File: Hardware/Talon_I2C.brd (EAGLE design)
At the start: 140 x 19 mm, 88 parts, among them J1 CONN_TALON_REMOTE, J2 CONN_SDI-12_LOGGERM8_TE_BOARD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, J3 CONN_SDI-12_LOGGERM8_TE_BOARD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, J4 CONN_SDI-12_LOGGERM8_TE_BOARD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, J5 CONN_APOGEE_LOGGER, Q1 AO3419, Q2 2N7002, Q3 AO3419, Q4 2N7002, Q5 AO3419, Q6 2N7002, Q7 AO3419, Q8 2N7002, U1 SN74LVC1G00SC70, U10 SN74LVC1G3157SC70, U11 SN74LVC1G3157SC70, U12 SN74LVC1G3157SC70, U13 SN74LVC1G3157SC70, U14 LM2621, U15 MCP3221, U16 LMR62014SOT23, U17 TXS0102DCU, U18 FDC6330L, U2 SN74LVC2G241DCU, U26 MCP23018QFN, U28 74HC4852, U29 SN74AUP1T157DCK, U3 MAX9034TSSOP, U30 MCP3421A3, U31 PCA9536DFN, U4 INA4180A2, U5 CD4044, U6 SN74HC04, U7 SN74AC08, U8 SIP32431TDFN, U9 SN74LVC1G17DCK

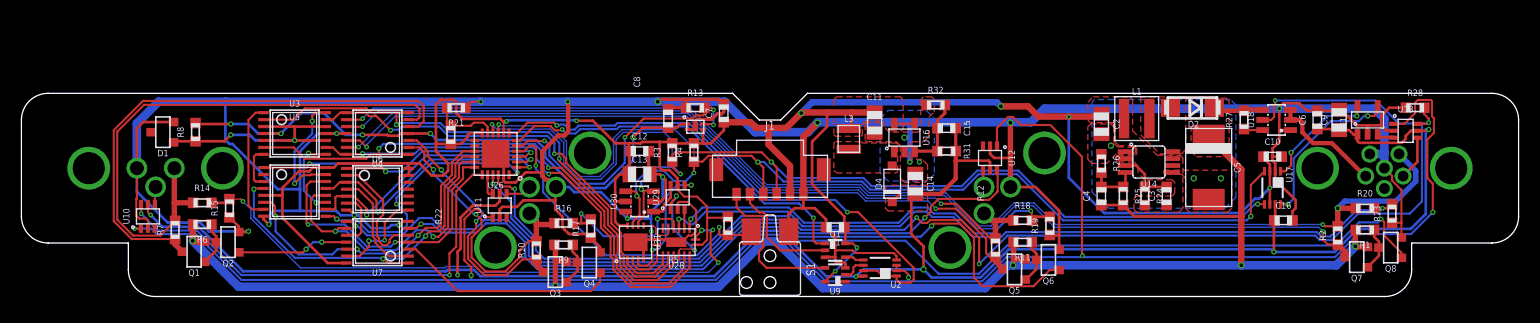
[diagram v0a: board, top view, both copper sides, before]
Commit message: Copper layout done
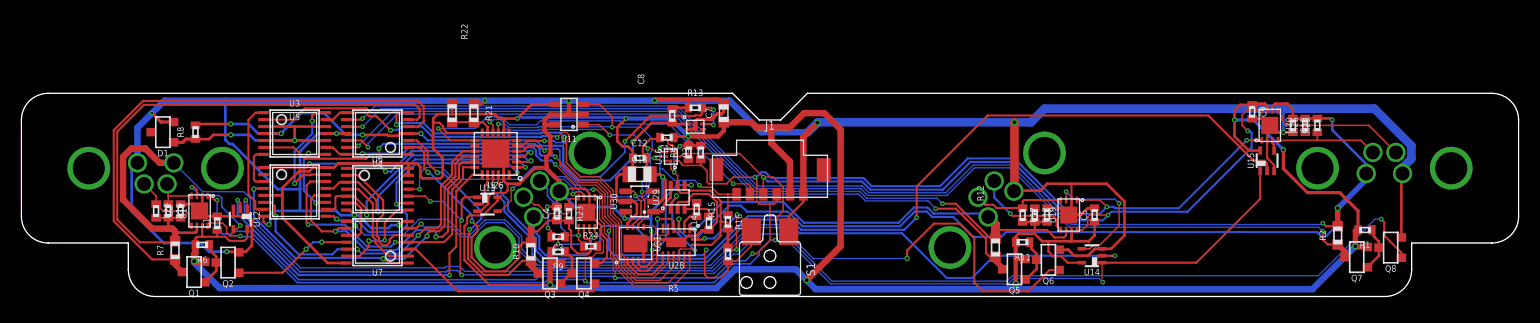
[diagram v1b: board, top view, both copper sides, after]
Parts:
- removed C14: 10uF, bschulz_passives:C0805
- removed C15: 220pF, bschulz_passives:C0603
- removed C16: 0.1uF, bschulz_passives:C0603
- removed D2: CDBA3100, bschulz:DO214AC
- removed D4: (no value), bschulz:SOD-123
- removed J2, J3, J4: CONN_SDI-12_LOGGERM8_TE_BOARDLOCK, GEMS_Plugs:1X03_M8_TE_T40410_BOARDLOCK
- removed J5: CONN_APOGEE_LOGGER, GEMS_Plugs:1X06_M8_PHOENIX_1456022_BOARDLOCK
- removed L1: 6.8uH, bschulz:WE-MAIA(4.1X4.1)
- removed L3: 10uH, bschulz:1008
- removed R27, R28: 100k, bschulz_passives:R0603
- removed R31: 40.2k, bschulz_passives:R0603
- removed R32: 13.3k, bschulz_passives:R0603
- removed U1: SN74LVC1G00SC70, bschulz:DCK_R-PDSO-G5
- removed U10: SN74LVC1G3157SC70, bschulz:DCK_R-PDSO-G6
- removed U2: SN74LVC2G241DCU, bschulz:DCU_(R-PDSO-G8)
- removed U9: SN74LVC1G17DCK, bschulz:DCK_R-PDSO-G5
- added J6, J7, J8, J9: CONN_I2C_LOGGER, GEMS_Plugs:1X04_M8_TE_T404103_BOARDLOCK
- added U19, U20: PCA9617WSON, bschulz:WSON-8_2X3
- C1, C10, C12, C3, C6, C8: device bschulz_passives:C0603 -> bschulz_passives:C0402
- C11: value 4.7uF -> 0.1uF; device bschulz_passives:C0805 -> bschulz_passives:C0402
- C2: value 22uF -> 0.1uF; device bschulz_passives:C0805 -> bschulz_passives:C0402
- C4: value (none) -> 0.1uF; device bschulz_passives:C0603 -> bschulz_passives:C0402
- C5: value 68uF -> 0.1uF; device bschulz_passives:C2917 -> bschulz_passives:C0402
- C9: value 10uF -> 0.1uF; device bschulz_passives:C0805 -> bschulz_passives:C0402
- R1, R11, R13, R14, R15, R17, R18, R19, R20, R23, R3, R4, R5, R6, R8, R9: device bschulz_passives:R0603 -> bschulz_passives:R0402
- R16: value (none) -> 100k; device bschulz_passives:R0603 -> bschulz_passives:R0402
- R24: value 470k -> (none); device bschulz_passives:R0603 -> bschulz_passives:R0402
- R25: value 115k -> (none); device bschulz_passives:R0603 -> bschulz_passives:R0402
- R26: value 13.3k -> (none); device bschulz_passives:R0603 -> bschulz_passives:R0402
- U11: value SN74LVC1G3157SC70 -> 24AA02SOT23; device bschulz:DCK_R-PDSO-G6 -> bschulz:SOT23-5
- U12, U13: value SN74LVC1G3157SC70 -> SN74AUP1G08DCK; device bschulz:DCK_R-PDSO-G6 -> bschulz:DCK_R-PDSO-G5
- U14: value LM2621 -> SN74AUP1G08DCK; device bschulz:DGK_S-PDSO-G8 -> bschulz:DCK_R-PDSO-G5
- U15: value MCP3221 -> SN74AUP1G08DCK; device bschulz:SOT23-5 -> bschulz:DCK_R-PDSO-G5
- U16: value LMR62014SOT23 -> FXMAR2102UMLP; device bschulz:DBV0005A -> bschulz:UQFN-8_1.4X1.2
- U17: value TXS0102DCU -> PCA9617WSON; device bschulz:DCU_(R-PDSO-G8) -> bschulz:WSON-8_2X3
- U18: value FDC6330L -> PCA9617WSON; device bschulz:SOT23-6L -> bschulz:WSON-8_2X3
- moved R20 113.0 mm to (-57.4, 8.00), turned to 270 degrees
- moved U17 100.4 mm to (-53.3, 8.00)
- moved C2 86.5 mm to (-55.1, 8.00), turned to 90 degrees
- moved U13 86.1 mm to (-26.4, 8.64)
- moved R19 82.4 mm to (-56.3, 8.00), turned to 270 degrees
- moved R23 77.0 mm to (-18.8, 7.75), turned to 270 degrees
- moved U12 70.3 mm to (-49.5, 7.24)
- moved U18 65.1 mm to (-17.1, 7.87), turned to 180 degrees
- moved C1 57.8 mm to (-51.7, 6.86), turned to 90 degrees
- moved C3 57.0 mm to (-19.8, 5.59), turned to 180 degrees
- moved R24 52.0 mm to (-16.8, 4.70), turned to 0 degrees
- moved C4 51.0 mm to (-19.9, 7.75)
- moved R14 47.4 mm to (-5.71, 6.86), turned to 90 degrees
- moved R15 43.7 mm to (-6.86, 8.13), turned to 270 degrees
- moved R17 40.4 mm to (23.6, 7.62), turned to 270 degrees
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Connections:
- removed net !RX: U2.6, U9.2
- removed net 12V: C4.1, C5.+, D2.C, Q1.2, Q3.2, Q5.2, Q7.2, R1.2, R11.2, R25.2, R27.2, R6.2, R9.2, U18.4
- removed net 5V: C14.1, C15.1, C16.1, C6.1, C9.1, D4.CAT, R31.2, U10.5, U11.5, U12.5, U13.5, U15.1, U17.7, U2.8
- removed net DATA: U10.1, U11.1, U12.1, U13.1, U2.2, U2.3
- removed net DATA_EN1: U10.6, U26.19
- removed net DATA_EN2: U11.6, U26.20
- removed net DATA_EN3: U12.6, U26.21
- removed net DATA_EN4: R28.2, U13.6, U18.5, U26.22
- removed net DATA_OUT1: J2.4, U10.4
- removed net DATA_OUT2: J3.4, U11.4
- removed net DATA_OUT3: J4.4, U12.4
- removed net DATA_OUT4: J5.3, U13.4
- removed net DATA_SENSE4: U13.3, U15.3
- removed net DIR: U2.1, U2.7, U26.7
- removed net FOUT: U1.1, U26.6
- removed net N$10: C15.2, R31.1, R32.2, U16.3
- removed net N$11: R27.1, U18.6
- removed net N$18: U28.3, U29.3
- removed net N$7: C3.2, R24.1, U14.3
- removed net N$8: D2.A, L1.P$2, U14.8
- removed net N$9: C4.2, R25.1, R26.2, U14.4
- removed net RX: J1.1, U9.4
- removed net SCL_HV: U15.5, U17.1
- removed net SDA_HV: U15.4, U17.8
- removed net SW1: D4.ANODE, L3.2, U16.1
- removed net TX: J1.2, U1.2
- removed net VHEATER: J5.5, U18.2, U18.3
- removed net VPORT1_OUT_SENSE: R14.2, R15.2, U28.1
- removed net VPORT2_OUT_SENSE: R16.2, R17.2, U28.5
- removed net VPORT3_OUT_SENSE: R18.2, R19.2, U28.2
- removed net VPORT4_OUT_SENSE: R20.2, R23.2, U28.4
- new net !I2C_OB_EN: U12.1, U13.1, U14.1, U15.1, U6.10
- new net DATA1_EN: U12.2, U26.19
- new net DATA1_EN_LOCAL: U12.4, U17.3
- new net DATA2_EN: U13.2, U26.20
- new net DATA2_EN_LOCAL: U13.4, U18.3
- new net DATA3_EN: U14.2, U26.21
- new net DATA3_EN_LOCAL: U14.4, U19.3
- new net DATA4_EN: U15.2, U26.22
- new net DATA4_EN_LOCAL: U15.4, U20.3
- new net I2C_OB_EN: J1.1, R16.1, U16.5, U6.11
- new net INTB: J1.2, U26.13
- new net N$6: R14.2, R15.1, U29.3
- new net PORT1_SCL: J6.4, R20.1, U17.5
- new net PORT1_SDA: J6.2, R19.1, U17.4
- new net PORT2_SCL: J7.4, R24.1, U18.5
- new net PORT2_SDA: J7.2, R23.1, U18.4
- new net PORT3_SCL: J8.4, R18.1, U19.5
- new net PORT3_SDA: J8.2, R17.1, U19.4
- new net PORT4_SCL: J9.4, R26.1, U20.5
- new net PORT4_SDA: J9.2, R25.1, U20.4
- new net SCL_OB: U11.1, U16.6, U26.9, U30.3, U31.6
- new net SDA_OB: U11.3, U16.7, U26.10, U30.4, U31.7
- net 3V3: now also C5.1, C9.1, Q1.2, Q3.2, Q5.2, Q7.2, R1.2, R11.2, R16.2, R6.2, R9.2, U11.4, U12.5, U13.5, U14.5, U15.5, U16.1, U16.8, U17.7, U18.7, U19.7, U20.7; no longer C10.1, C2.1, L1.P$1, L3.1, R24.2, U1.5, U14.2, U14.6, U14.7, U16.4, U16.5, U17.3, U17.6, U6.11, U9.5
- net GND: now also C3.2, C4.2, C5.2, J6.3, J7.3, J8.3, J9.3, R14.1, U11.5, U12.3, U13.3, U14.3, U15.3, U16.4, U17.EP, U18.2, U18.EP, U19.2, U19.EP, U20.2, U20.EP; no longer C14.2, C16.2, C5.-, J2.3, J3.3, J4.3, J5.1, J5.6, R15.1, R17.1, R19.1, R23.1, R26.1, R28.1, R32.1, U1.3, U10.2, U12.2, U13.2, U14.1, U14.5, U15.2, U16.2, U18.1, U2.4, U9.3
- net N$5: now also R15.2, U28.3; no longer U1.4, U2.5
- net SCL: now also U16.3, U17.8, U18.8, U19.8, U20.8; no longer U17.4, U26.9, U30.3, U31.6
- net SDA: now also U16.2, U17.1, U18.1, U19.1, U20.1; no longer U17.5, U26.10, U30.4, U31.7
- net VPORT1_OUT: now also C2.1, J6.1, R19.2, R20.2, U17.6, U28.1; no longer J2.1, R14.1
- net VPORT2_OUT: now also C4.1, J7.1, R23.2, R24.2, U18.6, U28.5; no longer J3.1, R16.1
- net VPORT3_OUT: now also C6.1, J8.1, R17.2, R18.2, U19.6, U28.2; no longer J4.1, R18.1
- net VPORT4_OUT: now also C10.1, J9.1, R25.2, R26.2, U20.6, U28.4; no longer J5.2, R20.1
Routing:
- net 5V: track 187.7 -> 0.00 mm, vias 6 -> 0
- net DATA: track 179.0 -> 0.00 mm, vias 5 -> 0
- net 12V: track 160.8 -> 0.00 mm, vias 5 -> 0
- net 3V3: track 210.9 -> 354.7 mm, vias 8 -> 14
- net DATA_EN4: track 129.3 -> 0.00 mm, vias 5 -> 0
- net !I2C_OB_EN: track 0.00 -> 125.2 mm, vias 0 -> 5
- net DATA4_EN: track 0.00 -> 88.1 mm, vias 0 -> 2
- net VPORT1_OUT: track 53.1 -> 135.5 mm, vias 0 -> 3
- net VPORT4_OUT: track 114.4 -> 189.3 mm, vias 3 -> 5
- net VPORT4_OUT_SENSE: track 72.7 -> 0.00 mm, vias 2 -> 0
- net DATA3_EN: track 0.00 -> 69.7 mm, vias 0 -> 2
- net DATA_EN3: track 59.0 -> 0.00 mm, vias 2 -> 0
- net VPORT1_OUT_SENSE: track 57.0 -> 0.00 mm, vias 4 -> 0
- net DIR: track 51.1 -> 0.00 mm, vias 2 -> 0
- net DATA_EN1: track 43.2 -> 0.00 mm, vias 2 -> 0
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- removed copper zone on layer 1, net 12V
- removed copper zone on layer 1, net 3V3
- removed copper zone on layer 1, net 5V
- removed copper zone on layer 1, net GND
- removed copper zone on layer 16, net GND
- removed copper zone on layer 1, net N$8
- removed copper zone on layer 1, net SW1
